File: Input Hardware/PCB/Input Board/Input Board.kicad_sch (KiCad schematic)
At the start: 4 parts

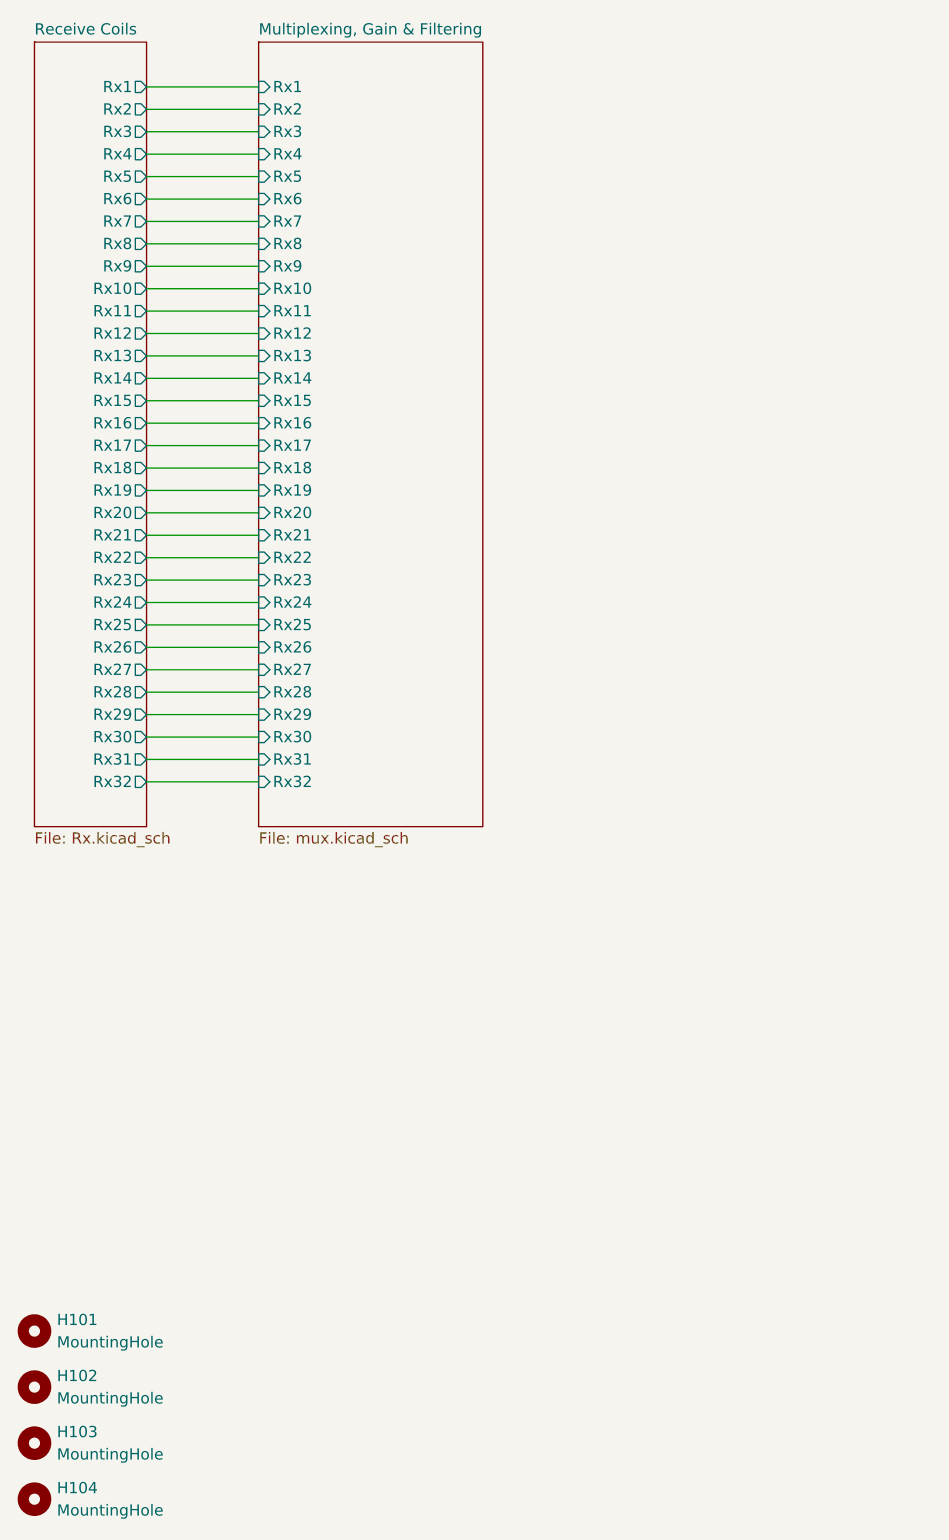
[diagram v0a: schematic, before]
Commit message: Progress
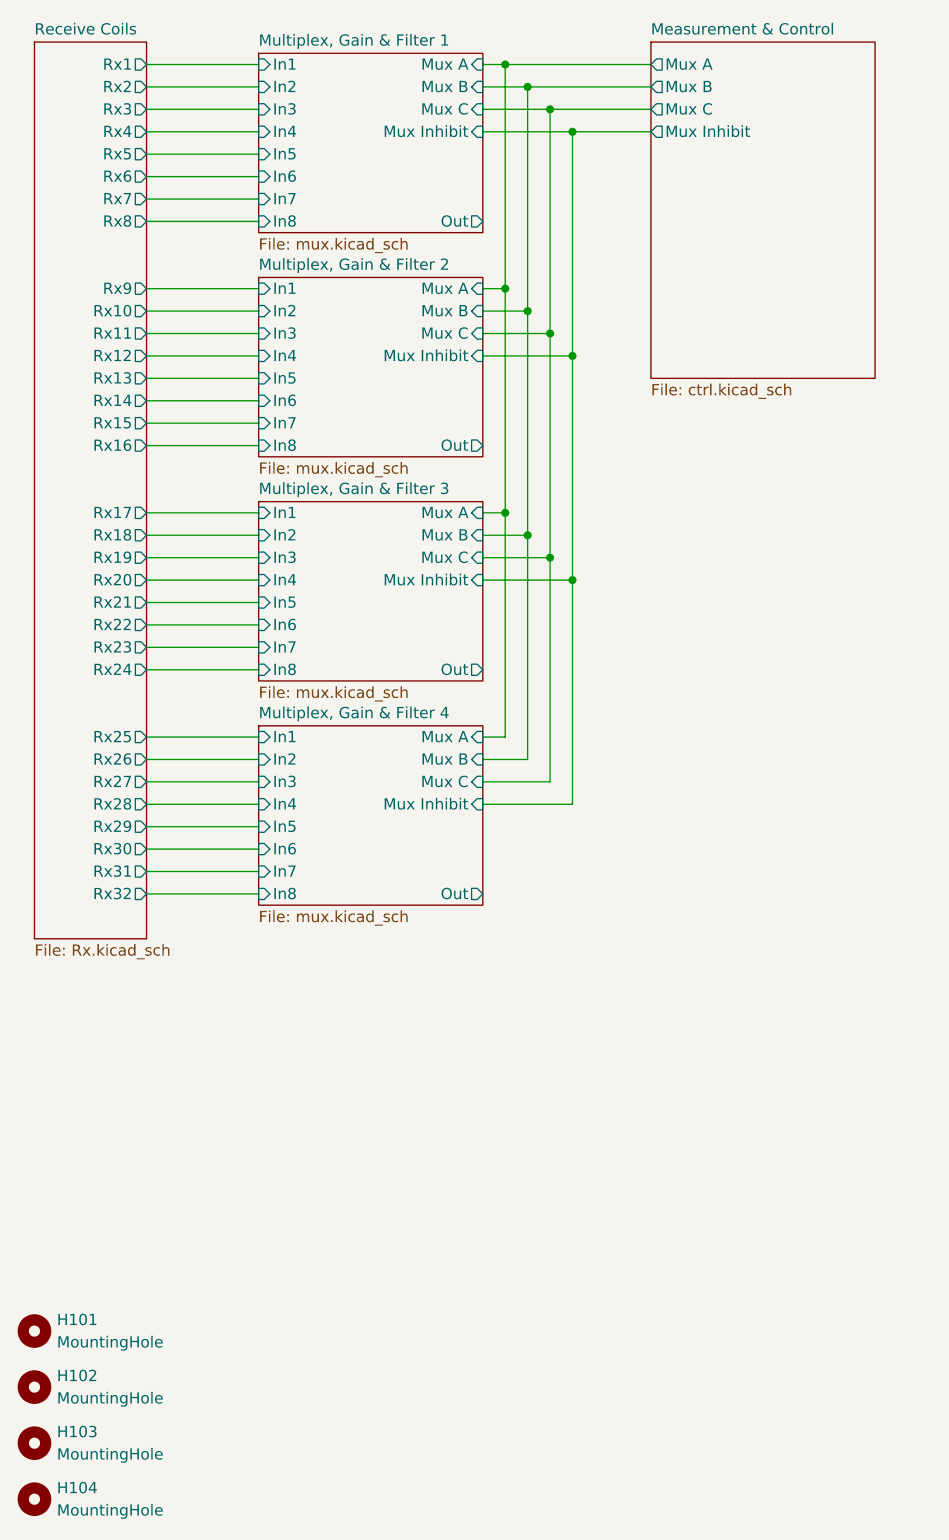
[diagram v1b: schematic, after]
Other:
- sheet Multiplexing, Gain & Filtering renamed Multiplex, Gain & Filter 1
- added sheet Measurement & Control (ctrl.kicad_sch)
- added sheet Multiplex, Gain & Filter 2 (mux.kicad_sch)
- added sheet Multiplex, Gain & Filter 3 (mux.kicad_sch)
- added sheet Multiplex, Gain & Filter 4 (mux.kicad_sch)
- sheet Multiplex, Gain & Filter 1 ports: added In1, In2, In3, In4, In5, In6, In7, In8, Mux A, Mux B, Mux C, Mux Inhibit, Out; removed Rx1, Rx10, Rx11, Rx12, Rx13, Rx14, Rx15, Rx16, Rx17, Rx18, Rx19, Rx2, Rx20, Rx21, Rx22, Rx23, Rx24, Rx25, Rx26, Rx27, Rx28, Rx29, Rx3, Rx30, Rx31, Rx32, Rx4, Rx5, Rx6, Rx7, Rx8, Rx9

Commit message: Fix Name
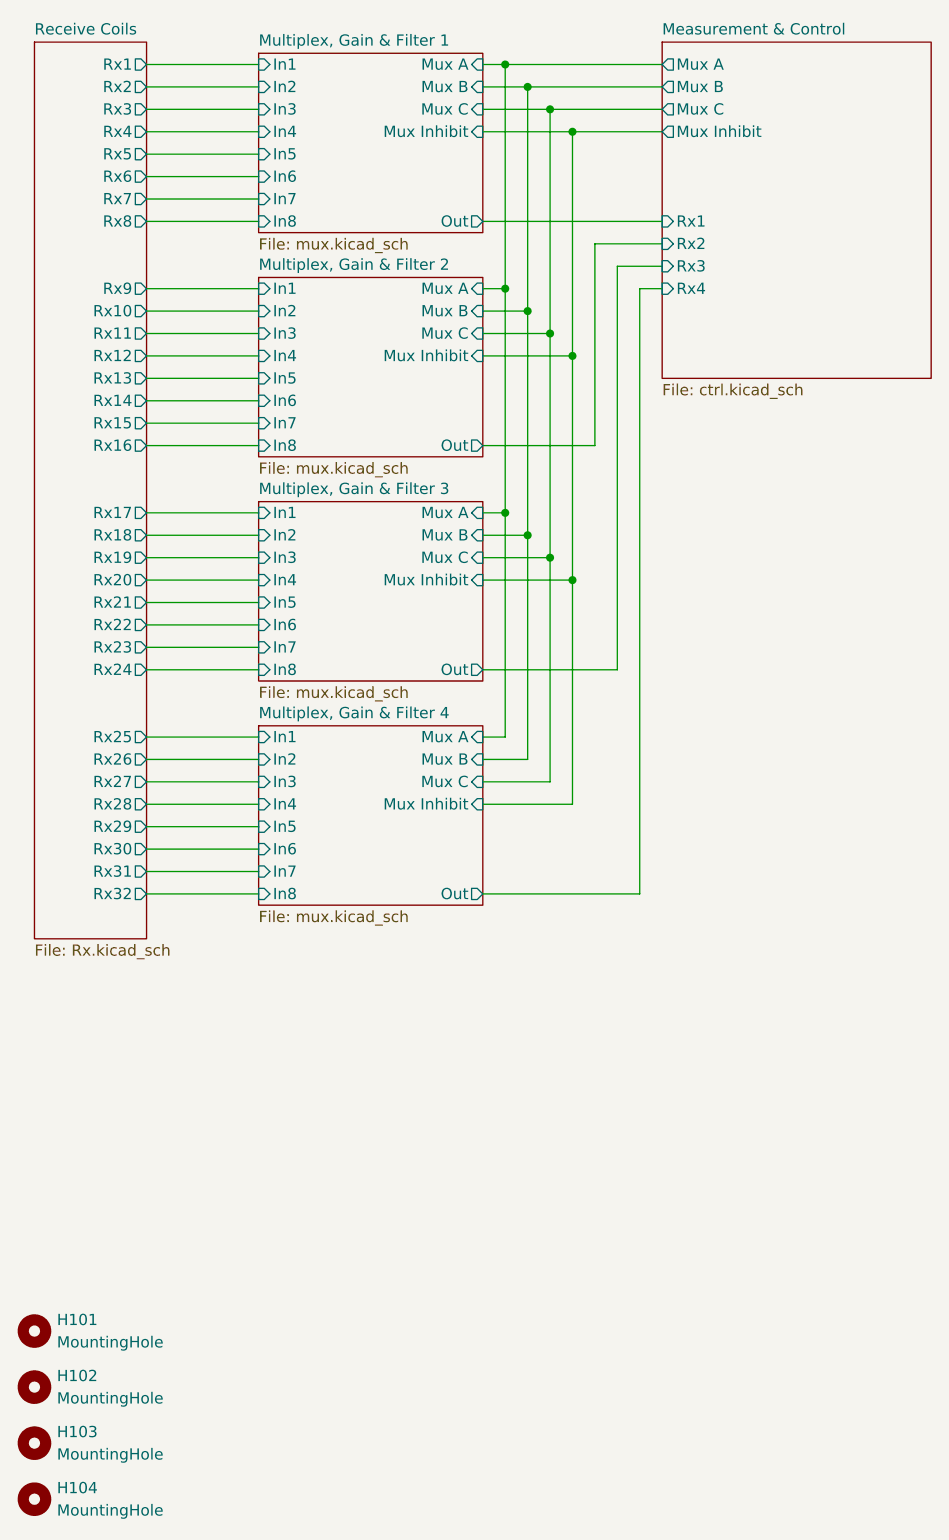
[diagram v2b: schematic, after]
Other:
- sheet Measurement & Control ports: added Rx1, Rx2, Rx3, Rx4; removed none
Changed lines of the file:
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@@
+	(wire
+		(pts
+			(xy 88.9 71.12) (xy 88.9 48.26)
+		)
+		(stroke
+			(width 0)
+			(type default)
+		)
+	)
 	(wire
 		(pts
@@
 	(wire
 		(pts
+			(xy 76.2 121.92) (xy 93.98 121.92)
+		)
+		(stroke
+			(width 0)
+			(type default)
+		)
+	)
+	(wire
+		(pts
 			(xy 76.2 78.74) (xy 78.74 78.74)
 		)
@@
 	(wire
 		(pts
-			(xy 86.36 35.56) (xy 95.25 35.56)
-		)
-		(stroke
-			(width 0)
-			(type default)
-		)
-	)
-	(wire
-		(pts
-			(xy 78.74 27.94) (xy 95.25 27.94)
+			(xy 86.36 35.56) (xy 96.52 35.56)
+		)
+		(stroke
+			(width 0)
+			(type default)
+		)
+	)
+	(wire
+		(pts
+			(xy 78.74 27.94) (xy 96.52 27.94)
 		)
 		(stroke
@@
 	(wire
 		(pts
-			(xy 83.82 33.02) (xy 95.25 33.02)
+			(xy 83.82 33.02) (xy 96.52 33.02)
 		)
 		(stroke
@@
 	(wire
 		(pts
+			(xy 76.2 96.52) (xy 91.44 96.52)
+		)
+		(stroke
+			(width 0)
+			(type default)
+		)
+	)
+	(wire
+		(pts
 			(xy 38.1 119.38) (xy 50.8 119.38)
 		)
@@
 	(wire
 		(pts
+			(xy 91.44 50.8) (xy 96.52 50.8)
+		)
+		(stroke
+			(width 0)
+			(type default)
+		)
+	)
+	(wire
+		(pts
 			(xy 76.2 35.56) (xy 86.36 35.56)
 		)
@@
 	(wire
 		(pts
+			(xy 88.9 48.26) (xy 96.52 48.26)
+		)
+		(stroke
+			(width 0)
+			(type default)
+		)
+	)
+	(wire
+		(pts
 			(xy 38.1 60.96) (xy 50.8 60.96)
 		)
@@
 	(wire
 		(pts
-			(xy 81.28 30.48) (xy 95.25 30.48)
+			(xy 93.98 121.92) (xy 93.98 53.34)
+		)
+		(stroke
+			(width 0)
+			(type default)
+		)
+	)
+	(wire
+		(pts
+			(xy 81.28 30.48) (xy 96.52 30.48)
 		)
 		(stroke
@@
 	(wire
 		(pts
+			(xy 91.44 96.52) (xy 91.44 50.8)
+		)
+		(stroke
+			(width 0)
+			(type default)
+		)
+	)
+	(wire
+		(pts
+			(xy 76.2 45.72) (xy 96.52 45.72)
+		)
+		(stroke
+			(width 0)
+			(type default)
+		)
+	)
+	(wire
+		(pts
 			(xy 76.2 81.28) (xy 81.28 81.28)
 		)
@@
 	(wire
 		(pts
+			(xy 76.2 71.12) (xy 88.9 71.12)
+		)
+		(stroke
+			(width 0)
+			(type default)
+		)
+	)
+	(wire
+		(pts
 			(xy 76.2 58.42) (xy 83.82 58.42)
 		)
@@
 		(pts
 			(xy 38.1 38.1) (xy 50.8 38.1)
+		)
+		(stroke
+			(width 0)
+			(type default)
+		)
+	)
+	(wire
+		(pts
+			(xy 93.98 53.34) (xy 96.52 53.34)
 		)
 		(stroke
@@
 	)
 	(sheet
-		(at 95.25 25.4)
-		(size 25.4 38.1)
+		(at 96.52 25.4)
+		(size 30.48 38.1)
 		(exclude_from_sim no)
 		(in_bom yes)
@@
 		)
 		(property "Sheetname" "Measurement & Control"
-			(at 95.25 24.6884 0)
+			(at 96.52 24.6884 0)
 			(effects
 				(font
@@
 		)
 		(property "Sheetfile" "ctrl.kicad_sch"
-			(at 95.25 64.0846 0)
+			(at 96.52 64.0846 0)
 			(effects
 				(font
@@
 		)
 		(pin "Mux A" output
-			(at 95.25 27.94 180)
+			(at 96.52 27.94 180)
 			(effects
 				(font
@@
 		)
 		(pin "Mux B" output
-			(at 95.25 30.48 180)
+			(at 96.52 30.48 180)
 			(effects
 				(font
@@
 		)
 		(pin "Mux C" output
-			(at 95.25 33.02 180)
+			(at 96.52 33.02 180)
 			(effects
 				(font
@@
 		)
 		(pin "Mux Inhibit" output
-			(at 95.25 35.56 180)
-			(effects
-				(font
+			(at 96.52 35.56 180)
+			(effects
+				(font
+					(size 1.27 1.27)
+				)
+				(justify left)
+			)
+		)
+		(pin "Rx1" input
+			(at 96.52 45.72 180)
+			(effects
+				(font
+					(size 1.27 1.27)
+				)
+				(justify left)
+			)
+		)
+		(pin "Rx2" input
+			(at 96.52 48.26 180)
+			(effects
+				(font
+					(size 1.27 1.27)
+				)
+				(justify left)
+			)
+		)
+		(pin "Rx3" input
+			(at 96.52 50.8 180)
+			(effects
+				(font
+					(size 1.27 1.27)
+				)
+				(justify left)
+			)
+		)
+		(pin "Rx4" input
+			(at 96.52 53.34 180)
+			(effects
+				(font
